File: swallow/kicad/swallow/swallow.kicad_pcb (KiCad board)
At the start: 2 copper layers, 85.1 x 69 mm, 35 parts, among them J1 Raspberry Pi 3/4 B, J10 evens, J2 echo2, J3 ground, J4 VCC, J5 echo3, J6 echo4, J7 echo1, J8 power terminal, J9 odds, SW1 SW_Push

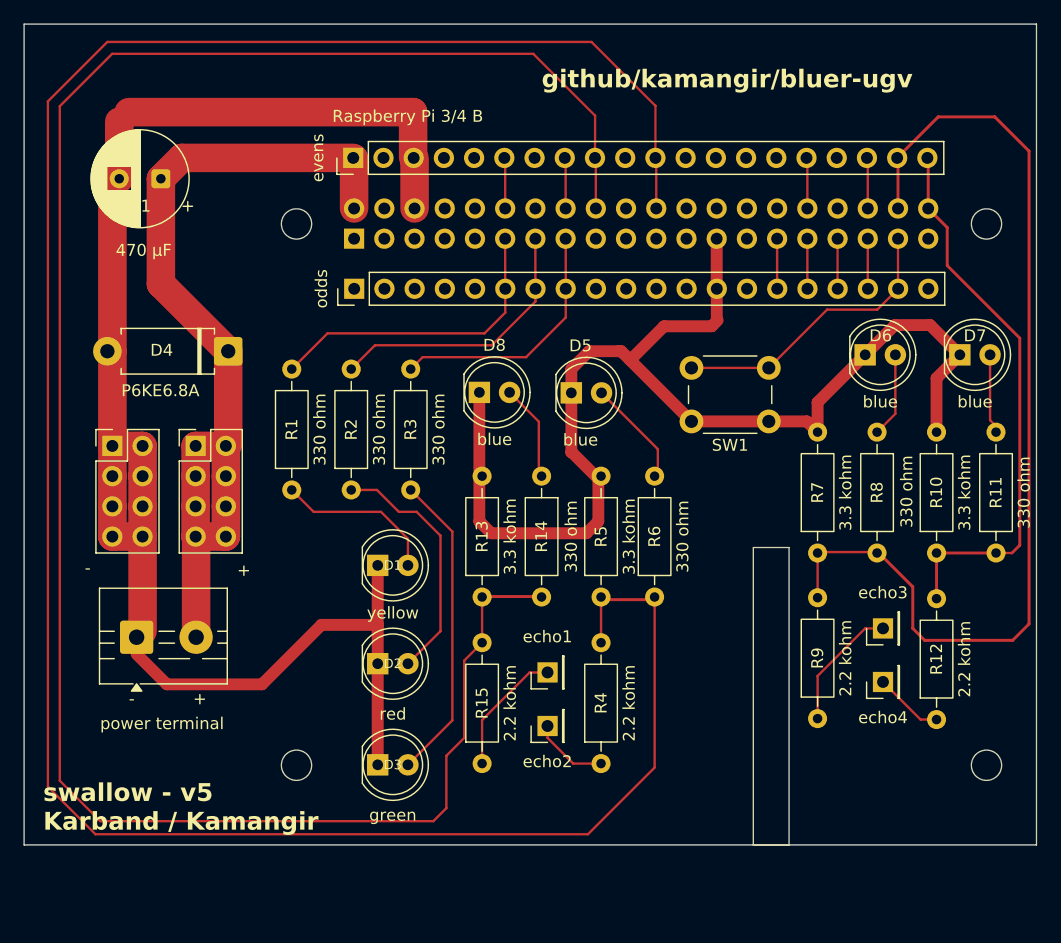
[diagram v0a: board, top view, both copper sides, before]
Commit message: ++ - kamangir/bolt#746
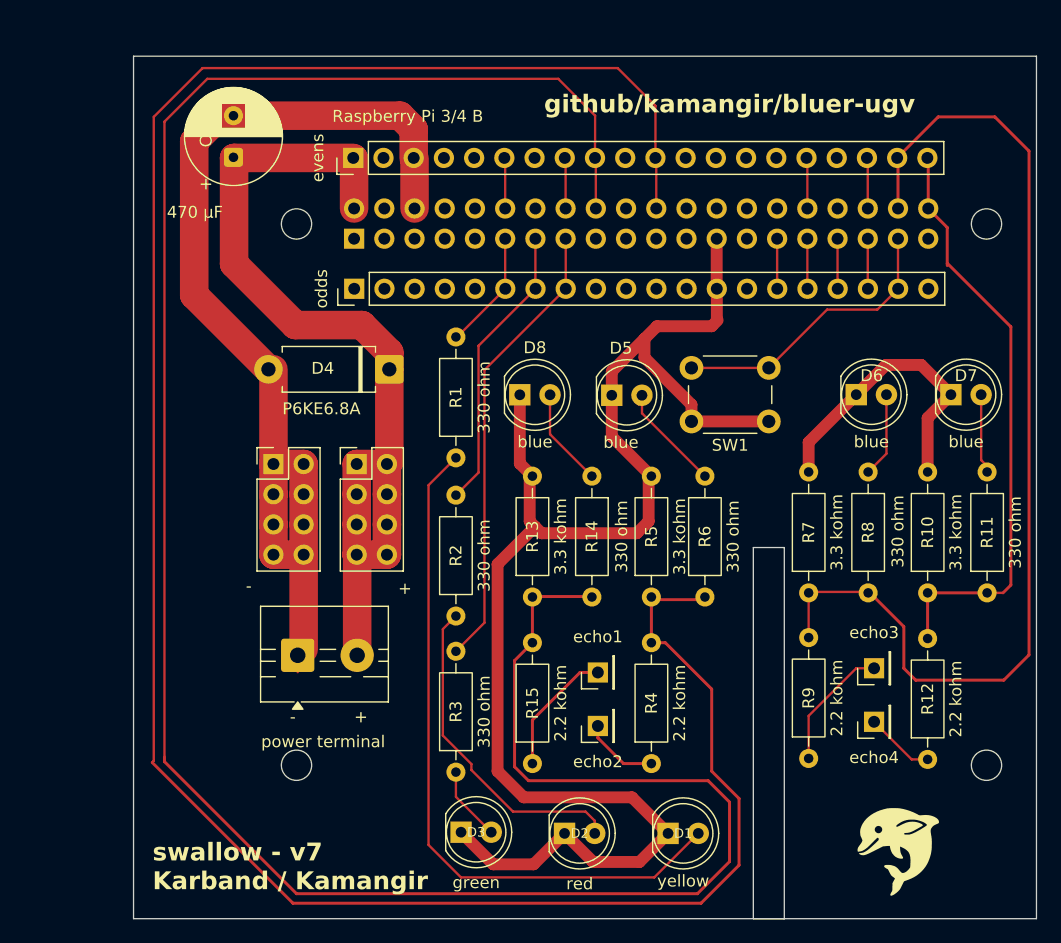
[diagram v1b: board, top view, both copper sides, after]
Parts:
- added REF**: orca-8mm, orca:orca-8mm, F.Cu at (183.5, 123.6)
- moved D1 33.2 mm to (164.1, 123.0)
- moved R3 24.0 mm to (146.3, 117.9)
- moved D2 21.2 mm to (155.4, 123.0)
- moved R1 14.1 mm to (146.3, 91.5)
- moved R2 13.8 mm to (146.3, 104.8)
- moved J3 13.6 mm to (131.0, 92.0)
- moved J4 13.6 mm to (138.0, 92.0)
- moved J8 13.6 mm to (133.0, 108.1)
- moved D4 13.6 mm to (140.7, 84.0)
- moved D3 9.01 mm to (146.7, 122.9)
- moved C1 6.36 mm to (127.6, 66.2), turned to 90 degrees
- moved J2 4.23 mm to (158.2, 114.0)
- moved J7 4.23 mm to (158.2, 109.5)
- moved R13 4.23 mm to (152.7, 103.2)
- moved R14 4.23 mm to (157.7, 93.0)
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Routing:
- net Net-(D1-A): track 13.7 -> 58.8 mm
- net Net-(J1-GPIO24): track 172.8 -> 199.0 mm
- net Net-(D3-A): track 26.1 -> 6.28 mm
- net Net-(J1-GPIO22): track 21.5 -> 38.5 mm
- net Net-(J1-GPIO17): track 26.1 -> 10.0 mm
- net Net-(D1-K): track 230.6 -> 239.9 mm
- net Net-(D2-A): track 21.0 -> 27.6 mm
- net Net-(J1-GPIO25): track 199.9 -> 195.1 mm
- net Net-(J1-GPIO20/MOSI1): track 85.2 -> 88.9 mm
- net Net-(J1-GPIO21/SCLK1): track 47.1 -> 50.3 mm
- net Net-(D4-K): track 74.9 -> 77.7 mm
- net Net-(J1-GPIO27): track 23.1 -> 24.3 mm
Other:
- board size 85.1 x 69 mm -> 75.9 x 72.5 mm
- board text added: "swallow - v7 Karband / Kamangir"
- board text removed: "swallow - v5 Karband / Kamangir"

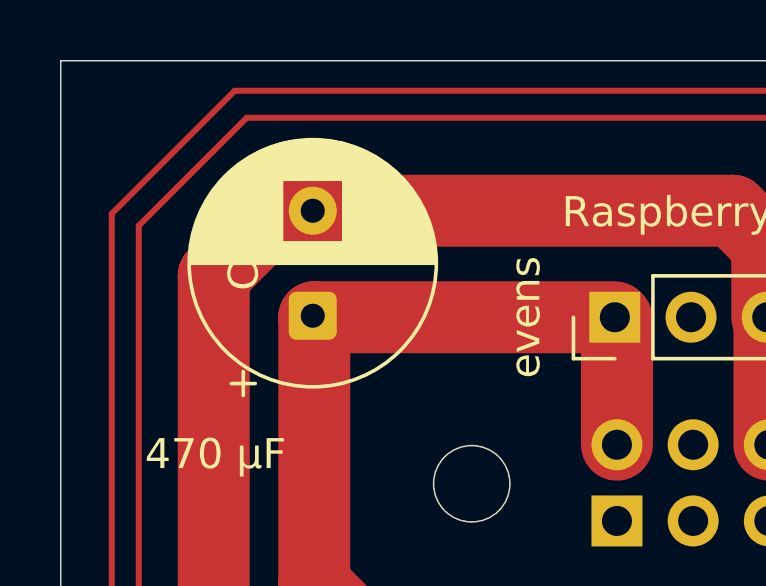
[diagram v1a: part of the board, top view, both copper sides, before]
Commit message: ++ - kamangir/bolt#746
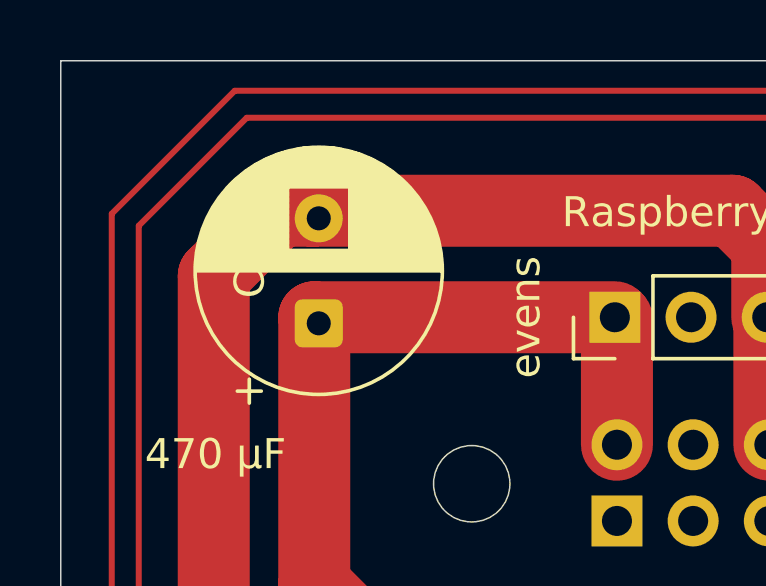
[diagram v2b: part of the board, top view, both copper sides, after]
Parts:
- moved C1 0.32 mm to (127.8, 66.5)
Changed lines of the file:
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@@
 	(footprint "Capacitor_THT:CP_Radial_D8.0mm_P3.50mm"
 		(layer "F.Cu")
-		(at 127.6 66.2 90)
+		(at 127.8 66.452651 90)
 		(descr "CP, Radial series, Radial, pin pitch=3.50mm, diameter=8mm, height=12mm, Electrolytic Capacitor")
 		(tags "CP Radial series Radial pin pitch 3.50mm diameter 8mm height 12mm Electrolytic Capacitor")

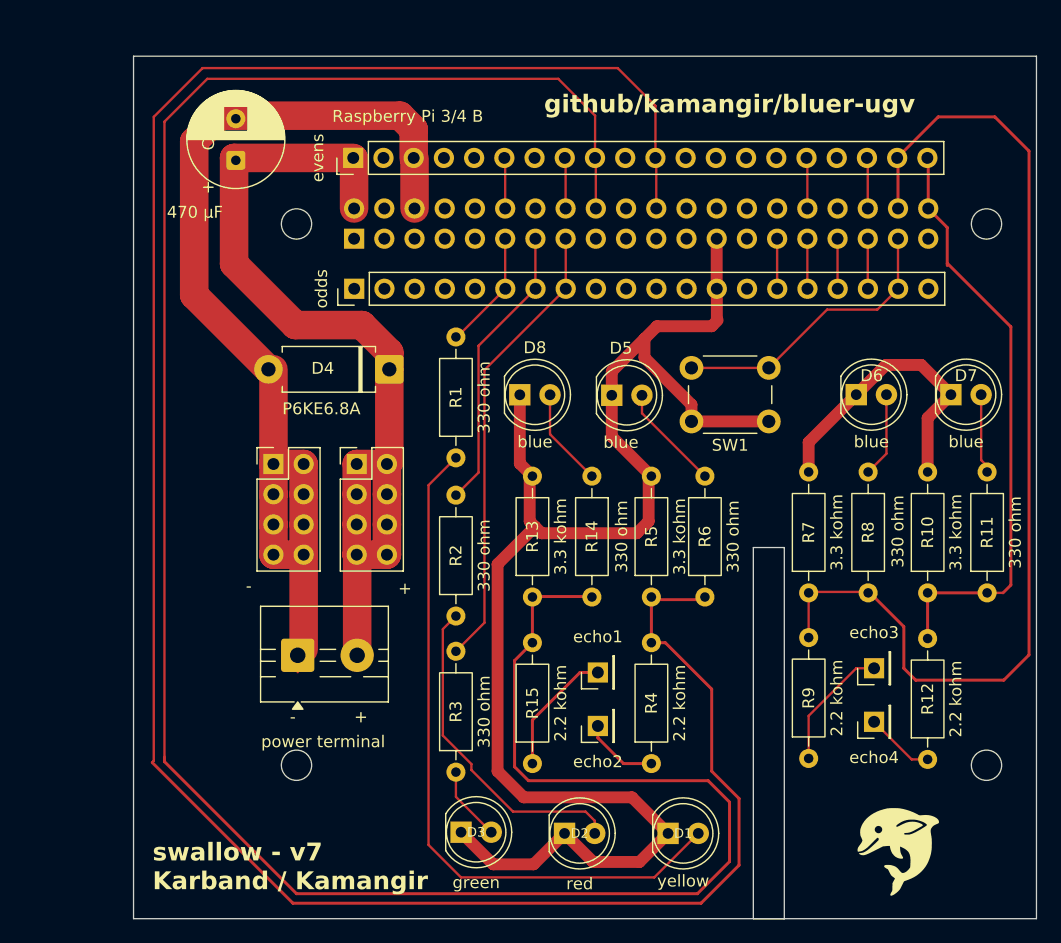
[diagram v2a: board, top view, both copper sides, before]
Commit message: ++ - kamangir/bolt#746
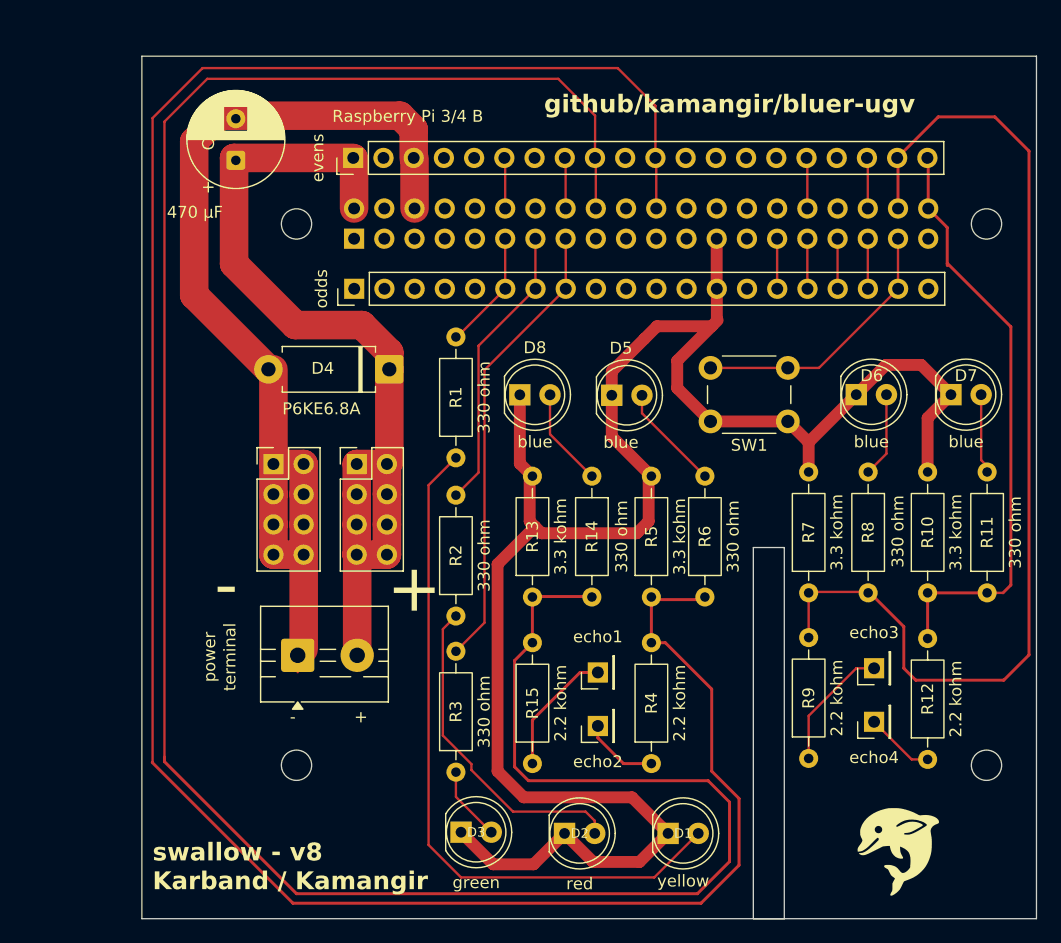
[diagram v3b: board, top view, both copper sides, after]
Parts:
- J8: value power terminal -> power
- moved SW1 1.60 mm to (174.2, 88.4)
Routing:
- net Net-(D1-K): track 239.9 -> 244.2 mm
- net Net-(J1-GPIO26): track 24.3 -> 22.7 mm
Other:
- board size 75.9 x 72.5 mm -> 75.2 x 72.5 mm
- board text added: "swallow - v8 Karband / Kamangir"
- board text added: "terminal"
- board text removed: "swallow - v7 Karband / Kamangir"
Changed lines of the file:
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@@
 			)
 		)
-		(property "Value" "power terminal"
-			(at 2.14 7.26 0)
+		(property "Value" "power"
+			(at -7.4 0.14 270)
 			(layer "F.SilkS")
 			(effects
@@
 	(footprint "Button_Switch_THT:SW_PUSH_6mm"
 		(layer "F.Cu")
-		(at 172.6 88.4 180)
+		(at 174.2 88.4 180)
 		(descr "Generic 6mm SW tactile push button")
 		(tags "tact sw push 6mm")
@@
 	)
 	(gr_rect
-		(start 119.2 57.7)
+		(start 119.9 57.7)
 		(end 195.1 130.2)
 		(stroke
@@
 	)
 	(gr_text "-"
-		(at 128.64 102.82 0)
+		(at 126 104.5 0)
 		(layer "F.SilkS")
 		(effects
 			(font
-				(size 1 1)
-				(thickness 0.1)
+				(size 4 4)
+				(thickness 0.2)
 			)
 			(justify left bottom)
@@
 		)
 	)
+	(gr_text "terminal"
+		(at 127.3 108.2 90)
+		(layer "F.SilkS")
+		(effects
+			(font
+				(size 1 1)
+				(thickness 0.15)
+			)
+		)
+	)
 	(gr_text "D4"
 		(at 134.14 84.52 0)
@@
 		)
 	)
-	(gr_text "swallow - v7\nKarband / Kamangir"
+	(gr_text "swallow - v8\nKarband / Kamangir"
 		(at 120.8 127.9 0)
 		(layer "F.SilkS")
@@
 	)
 	(gr_text "+"
-		(at 141.44 103.02 0)
+		(at 140.5 104.8 0)
 		(layer "F.SilkS")
 		(effects
 			(font
-				(size 1 1)
-				(thickness 0.1)
+				(size 4 4)
+				(thickness 0.2)
 			)
 			(justify left bottom)
@@
 		(layer "User.1")
 		(pts
-			(xy 171.3 124) (xy 119.2 124)
+			(xy 132.9 71.8) (xy 119.9 57.7)
+		)
+		(height -28)
+		(orientation 0)
+		(format
+			(prefix "")
+			(suffix "")
+			(units 3)
+			(units_format 0)
+			(precision 4)
+			(suppress_zeroes yes)
+		)
+		(style
+			(thickness 0.2)
+			(arrow_length 1.27)
+			(text_position_mode 2)
+			(arrow_direction outward)
+			(extension_height 0.58642)
+			(extension_offset 0.5)
+			(keep_text_aligned yes)
+		)
+		(gr_text "13"
+			(at 126.4 42 0)
+			(layer "User.1")
+			(effects
+				(font
+					(size 1 1)
+					(thickness 0.3)
+				)
+			)
+		)
+	)
+	(dimension
+		(type orthogonal)
+		(layer "User.1")
+		(pts
+			(xy 171.3 124) (xy 119.9 124)
 		)
 		(height 8.6)
@@
 			(keep_text_aligned yes)
 		)
-		(gr_text "52.1"
-			(at 145.25 131.45 0)
+		(gr_text "51.4"
+			(at 145.6 131.45 0)
 			(layer "User.1")
 			(effects
@@
 		(layer "User.1")
 		(pts
-			(xy 173.9 123.9) (xy 171.3 123.9)
+			(xy 192.172792 71.8) (xy 189.627208 71.8)
 		)
-		(height -2.7)
+		(height 9.8)
 		(orientation 0)
 		(format
@@
 			(units_format 0)
 			(precision 4)
+			(override_value "2.5")
 			(suppress_zeroes yes)
 		)
@@
 			(arrow_length 1.27)
 			(text_position_mode 0)
-			(arrow_direction outward)
+			(arrow_direction inward)
 			(extension_height 0.58642)
 			(extension_offset 0.5)
 			(keep_text_aligned yes)
 		)
-		(gr_text "2.6"
-			(at 172.6 120.05 0)
+		(gr_text "2.5"
+			(at 190.9 80.45 0)
 			(layer "User.1")
 			(effects
@@
 		(layer "User.1")
 		(pts
-			(xy 132.9 117.3) (xy 119.2 117.3)
+			(xy 173.9 123.9) (xy 171.3 123.9)
 		)
-		(height 26.5)
+		(height -2.7)
 		(orientation 0)
 		(format
@@
 		)
 		(style
-			(thickness 0.2)
+			(thickness 0.1)
 			(arrow_length 1.27)
 			(text_position_mode 0)
@@
 			(keep_text_aligned yes)
 		)
-		(gr_text "13.7"
-			(at 126.05 142.65 0)
+		(gr_text "2.6"
+			(at 172.6 120.05 0)
 			(layer "User.1")
 			(effects
@@
 			(xy 132.9 71.8) (xy 132.9 117.3)
 		)
-		(height -37.7)
+		(height -26.1)
 		(orientation 1)
 		(format
@@
 		)
 		(gr_text "45.5"
-			(at 94.05 94.55 90)
+			(at 105.65 94.55 90)
 			(layer "User.1")
 			(effects
@@
 		(layer "User.1")
 		(pts
-			(xy 119.2 124) (xy 195.1 124)
+			(xy 119.9 124) (xy 195.1 124)
 		)
 		(height 26.7)
@@
 			(keep_text_aligned yes)
 		)
-		(gr_text "75.9"
-			(at 157.15 149.6 0)
+		(gr_text "75.2"
+			(at 157.5 149.6 0)
 			(layer "User.1")
 			(effects
@@
 		(layer "User.1")
 		(pts
-			(xy 195.1 124) (xy 174.3 124)
+			(xy 195.1 124) (xy 173.9 124)
 		)
 		(height 8.6)
@@
 			(keep_text_aligned yes)
 		)
-		(gr_text "20.8"
-			(at 184.7 131.45 0)
+		(gr_text "21.2"
+			(at 184.5 131.45 0)
 			(layer "User.1")
 			(effects
@@
 	)
 	(segment
-		(start 166.1 88.4)
-		(end 166.1 86.985787)
-		(width 1)
-		(layer "F.Cu")
-		(net 1)
-	)
-	(segment
 		(start 157.83 125.43)
 		(end 161.73 125.43)
@@
 	)
 	(segment
+		(start 167.7 88.4)
+		(end 164.9 85.6)
+		(width 1)
+		(layer "F.Cu")
+		(net 1)
+	)
+	(segment
 		(start 168.22 77.24)
 		(end 168.23 77.25)
@@
 	)
 	(segment
-		(start 172.6 88.4)
-		(end 166.1 88.4)
+		(start 174.2 88.4)
+		(end 167.7 88.4)
 		(width 1)
 		(layer "F.Cu")
@@
 	)
 	(segment
-		(start 162.15 83.035787)
-		(end 162.15 81.45)
-		(width 1)
-		(layer "F.Cu")
-		(net 1)
-	)
-	(segment
 		(start 161.1 120)
 		(end 152 120)
@@
 	)
 	(segment
+		(start 164.9 85.6)
+		(end 164.9 83.3)
+		(width 1)
+		(layer "F.Cu")
+		(net 1)
+	)
+	(segment
 		(start 130.96 84.02)
 		(end 130.96 91.98)
@@
 	)
 	(segment
-		(start 166.1 86.985787)
-		(end 162.15 83.035787)
-		(width 1)
-		(layer "F.Cu")
-		(net 1)
-	)
-	(segment
 		(start 164.13 123.03)
 		(end 161.1 120)
@@
 	)
 	(segment
+		(start 175.95 90.15)
+		(end 174.2 88.4)
+		(width 1)
+		(layer "F.Cu")
+		(net 1)
+	)
+	(segment
 		(start 151.67 91.94)
 		(end 152.73 93)
@@
 	)
 	(segment
+		(start 164.9 83.3)
+		(end 167.8 80.4)
+		(width 1)
+		(layer "F.Cu")
+		(net 1)
+	)
+	(segment
 		(start 182.45 83.65)
 		(end 179.95 86.15)
@@
 	)
 	(segment
-		(start 183.46 77.24)
-		(end 183.47 77.25)
+		(start 176.82 83.9)
+		(end 174.2 83.9)
 		(width 0.2)
 		(layer "F.Cu")
@@
 	)
 	(segment
-		(start 183.46 73.04)
-		(end 183.46 77.24)
+		(start 183.46 77.24)
+		(end 183.47 77.25)
 		(width 0.2)
 		(layer "F.Cu")
@@
 	(segment
 		(start 183.47 77.25)
-		(end 181.72 79)
+		(end 176.82 83.9)
 		(width 0.2)
 		(layer "F.Cu")
@@
 	)
 	(segment
-		(start 181.72 79)
-		(end 177.5 79)
-		(width 0.2)
-		(layer "F.Cu")
-		(net 18)
-	)
-	(segment
-		(start 177.5 79)
-		(end 172.6 83.9)
+		(start 183.46 73.04)
+		(end 183.46 77.24)
 		(width 0.2)
 		(layer "F.Cu")
@@
 	)
 	(segment
-		(start 172.6 83.9)
-		(end 166.1 83.9)
+		(start 174.2 83.9)
+		(end 167.7 83.9)
 		(width 0.2)
 		(layer "F.Cu")
@@
 	)
 	(segment
-		(start 125 58.7)
-		(end 159.9 58.7)
-		(width 0.2)
-		(layer "F.Cu")
-		(net 58)
-	)
-	(segment
 		(start 163.14 70.5)
 		(end 163.14 66.32)
@@
 	)
 	(segment
+		(start 125 58.7)
+		(end 159.9 58.7)
+		(width 0.2)
+		(layer "F.Cu")
+		(net 58)
+	)
+	(segment
+		(start 120.8 117.0329)
+		(end 120.8 62.9)
+		(width 0.2)
+		(layer "F.Cu")
+		(net 58)
+	)
+	(segment
 		(start 167.5 103.38)
 		(end 162.5 103.38)
@@
 	)
 	(segment
+		(start 159.9 58.7)
+		(end 163.07 61.87)
+		(width 0.2)
+		(layer "F.Cu")
+		(net 58)
+	)
+	(segment
 		(start 162.73 107)
 		(end 162.73 103.16)
@@
 	)
 	(segment
+		(start 120.8 62.9)
+		(end 125 58.7)
+		(width 0.2)
+		(layer "F.Cu")
+		(net 58)
+	)
+	(segment
 		(start 163.14 66.32)
 		(end 163.07 66.25)
@@
 	)
 	(segment
-		(start 120.9 62.8)
-		(end 125 58.7)
-		(width 0.2)
-		(layer "F.Cu")
-		(net 58)
-	)
-	(segment
-		(start 120.76645 117.06645)
-		(end 120.9 116.9329)
-		(width 0.2)
-		(layer "F.Cu")
-		(net 58)
-	)
-	(segment
 		(start 163.07 61.87)
 		(end 163.07 66.25)
@@
 	)
 	(segment
-		(start 167.8 110.9)
-		(end 167.8 117.8)
-		(width 0.25)
-		(layer "F.Cu")
-		(net 58)
-	)
-	(segment
-		(start 159.9 58.7)
-		(end 163.07 61.87)
+		(start 120.76645 117.06645)
+		(end 120.8 117.0329)
 		(width 0.2)
 		(layer "F.Cu")
@@
 	)
 	(segment
-		(start 120.9 116.9329)
-		(end 120.9 62.8)
-		(width 0.2)
+		(start 167.8 110.9)
+		(end 167.8 117.8)
+		(width 0.25)
 		(layer "F.Cu")
 		(net 58)

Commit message: ++ - kamangir/bolt#746
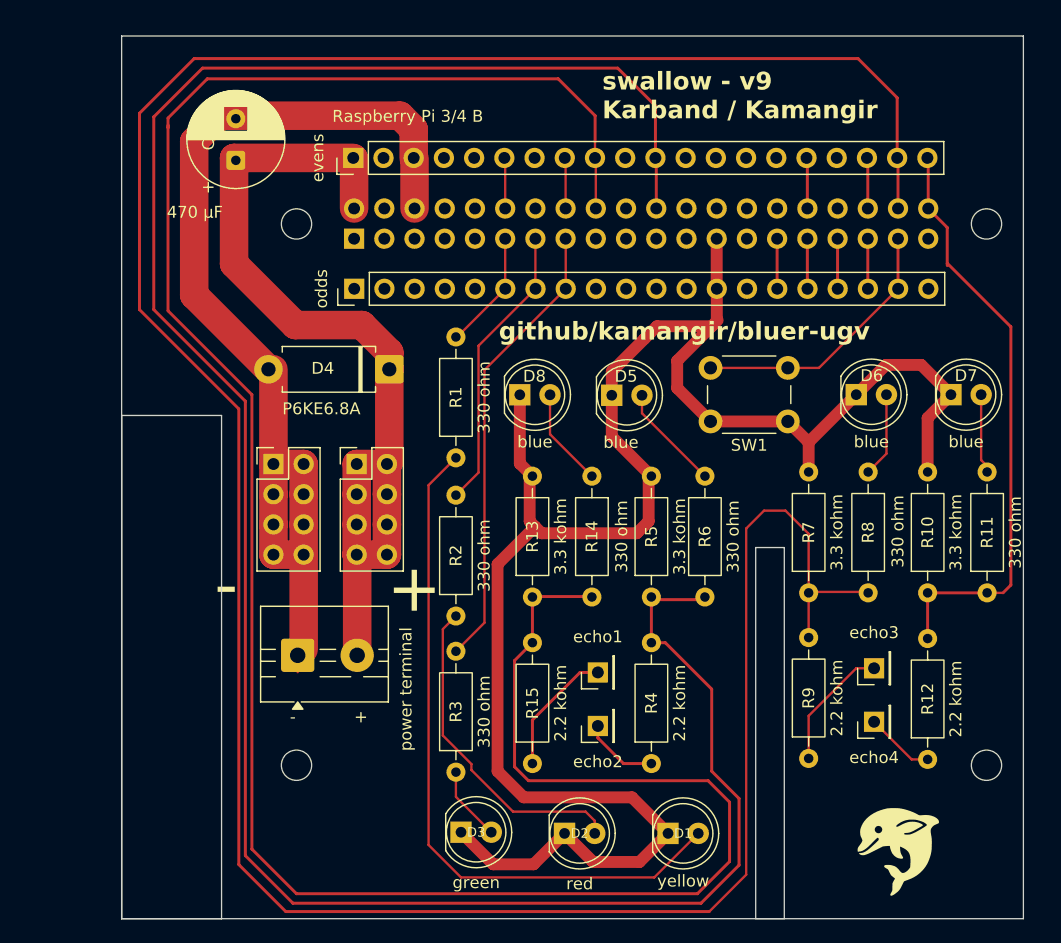
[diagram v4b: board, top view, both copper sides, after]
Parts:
- J8: value power -> power terminal
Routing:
- net Net-(J1-GPIO20/MOSI1): track 88.9 -> 238.2 mm
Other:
- board size 75.2 x 72.5 mm -> 75.8 x 74.2 mm
- board text added: "swallow - v9 Karband / Kamangir"
- board text removed: "swallow - v8 Karband / Kamangir"
- board text removed: "terminal"
